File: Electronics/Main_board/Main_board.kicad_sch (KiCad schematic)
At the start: 39 parts, among them Q1 S8050, Q2 S8050, Q3 IRFZ44n, Q4 IRFZ44n, Q5 IRFZ44n, U1 AMS1117-3.3, U2 NRF24L01_Breakout, U3 LM7805_TO220, U4 PC817, U5 PC817, U6 PC817

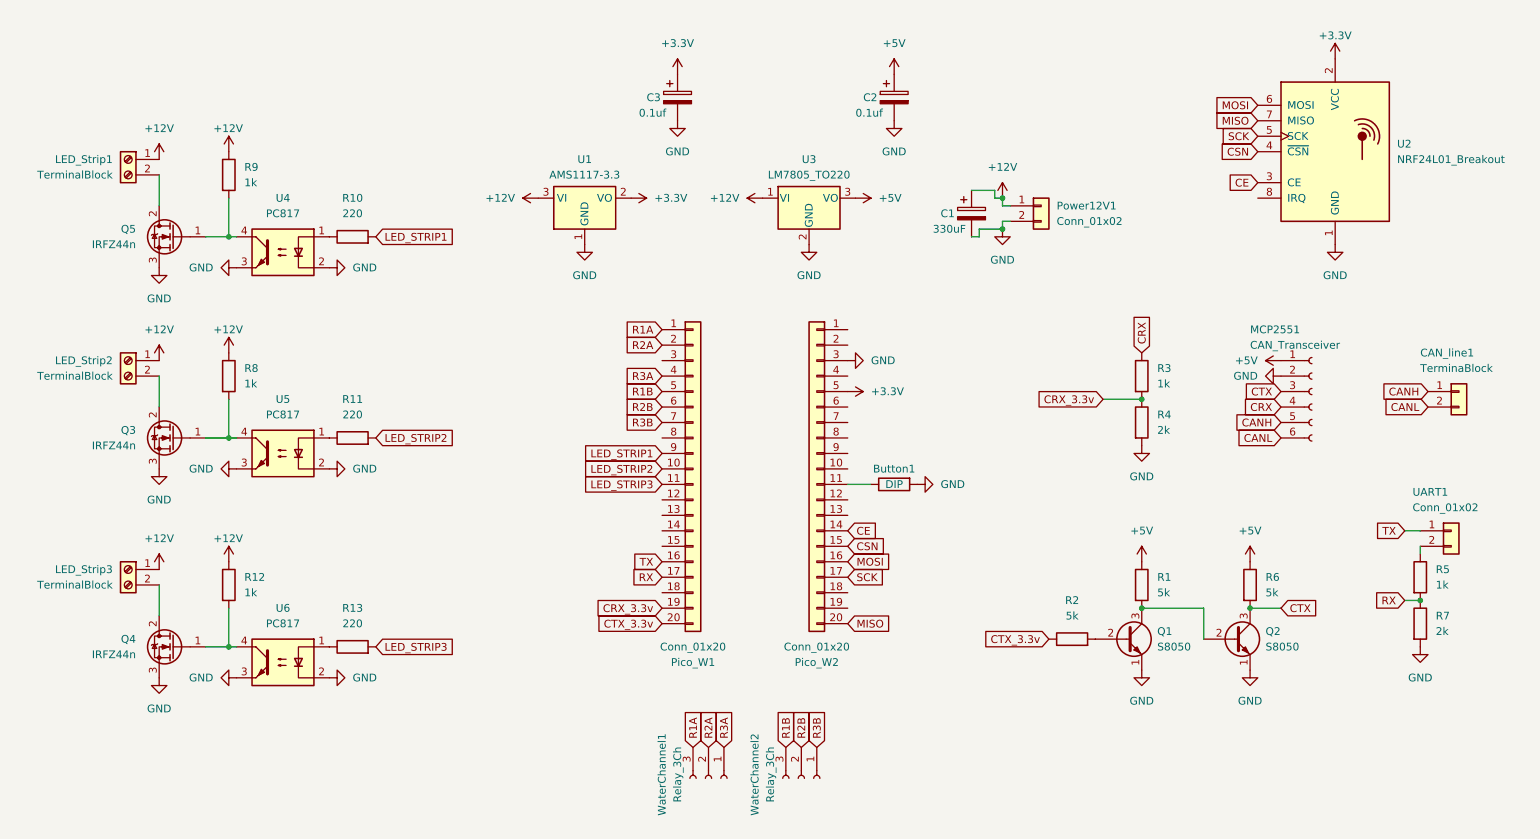
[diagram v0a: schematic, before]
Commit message: finished Main Board PCB
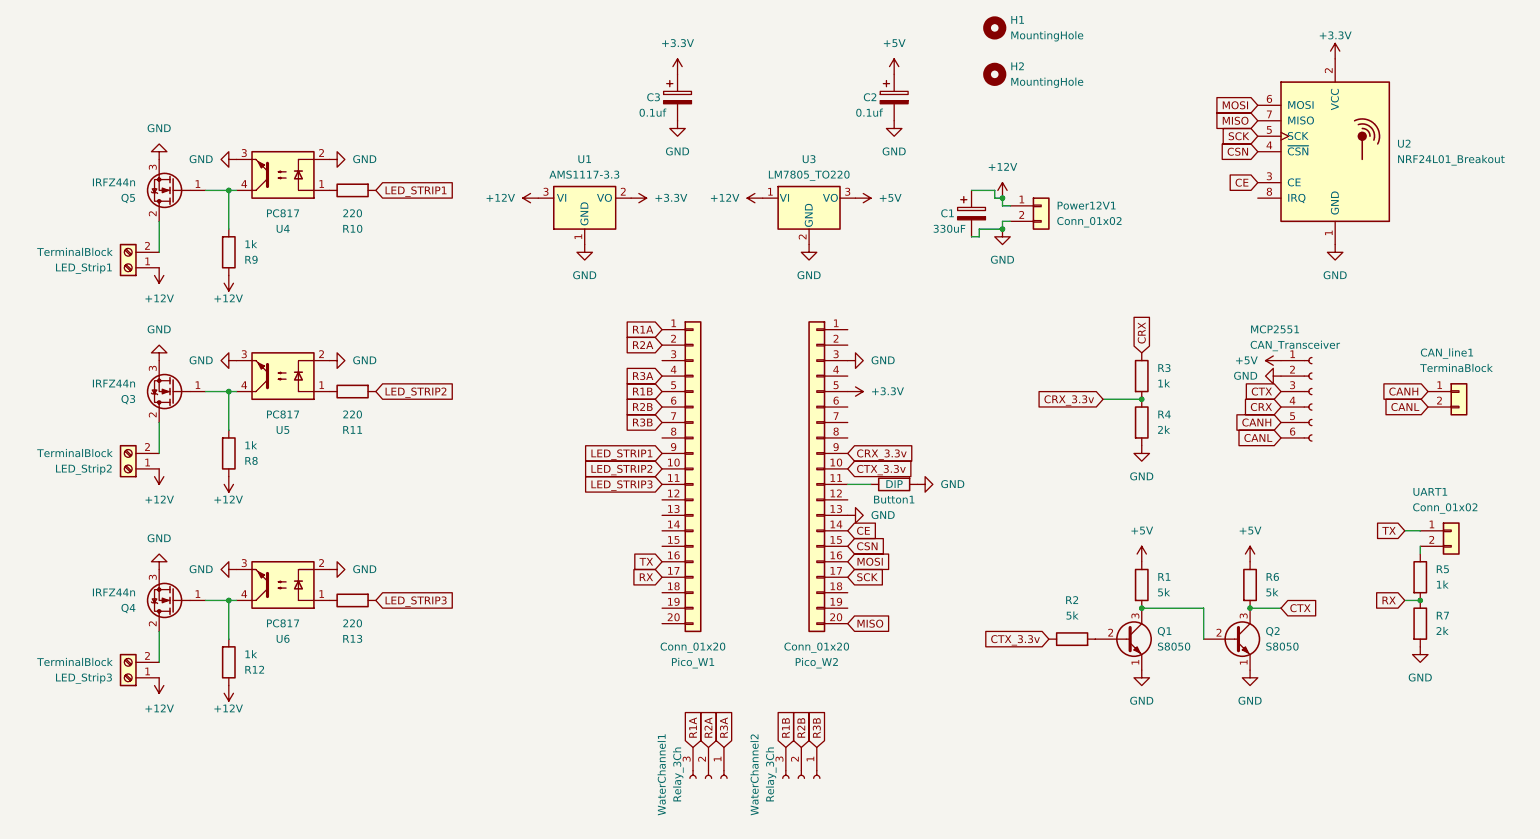
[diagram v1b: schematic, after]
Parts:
- added H1, H2: MountingHole, MountingHole:MountingHole_3.2mm_M3_DIN965_Pad_TopBottom, symbol Mechanical:MountingHole
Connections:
- net CRX_3.3v: now also Pico_W2.9 (Pin_9); no longer Pico_W1.19 (Pin_19)
- net CTX_3.3v: now also Pico_W2.10 (Pin_10); no longer Pico_W1.20 (Pin_20)
- net GND: now also Pico_W2.13 (Pin_13)
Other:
- moved on the sheet: LED_Strip1, LED_Strip2, LED_Strip3, Q3, Q4, Q5, R10, R11, R12, R13, R8, R9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
